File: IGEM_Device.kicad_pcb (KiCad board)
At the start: 2 copper layers, 50.2 x 47 mm, 28 parts, among them J1 67997-410HLF, J2 Electrode_Conn, J3 Batt_Conn, SW1 Power_Switch, U1 SaBLE-X-R2, U2 TC1014-2.85VCT713, U3 LMP91000SD_NOPB, U4 LM334MX_NOPB, U5 TPS79718QDCKRQ1, U6 G-NIMO-003

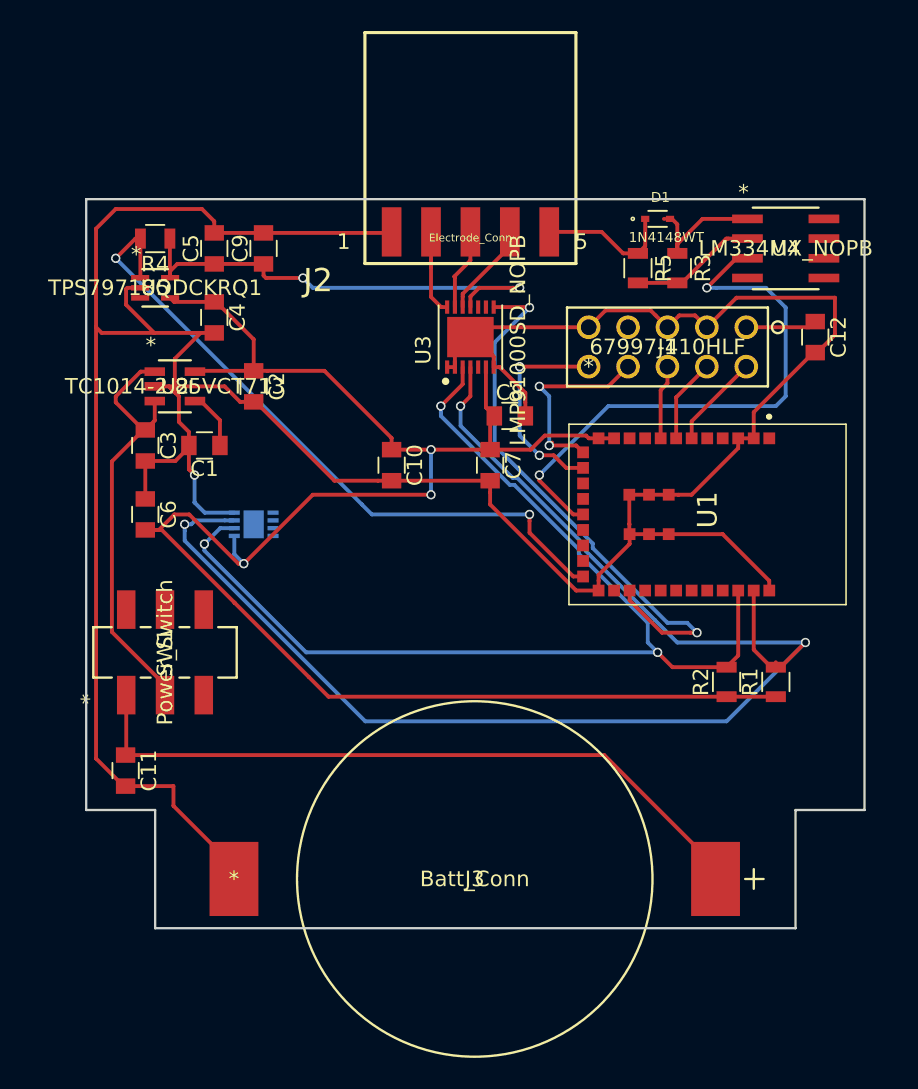
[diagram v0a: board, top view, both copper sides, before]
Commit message: Minor changes
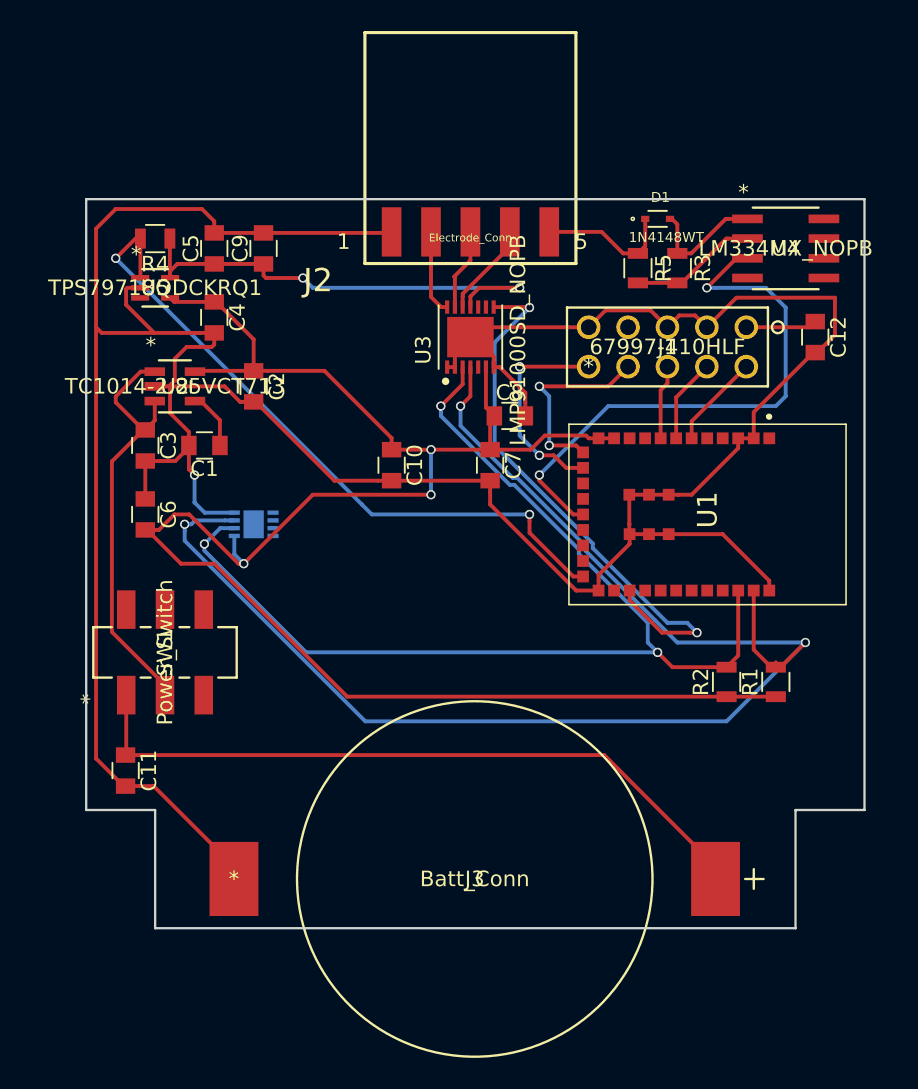
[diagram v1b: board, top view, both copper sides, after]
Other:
- rule via_min_size: 0.4 -> 0.5
